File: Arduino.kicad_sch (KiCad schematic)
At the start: 1 part

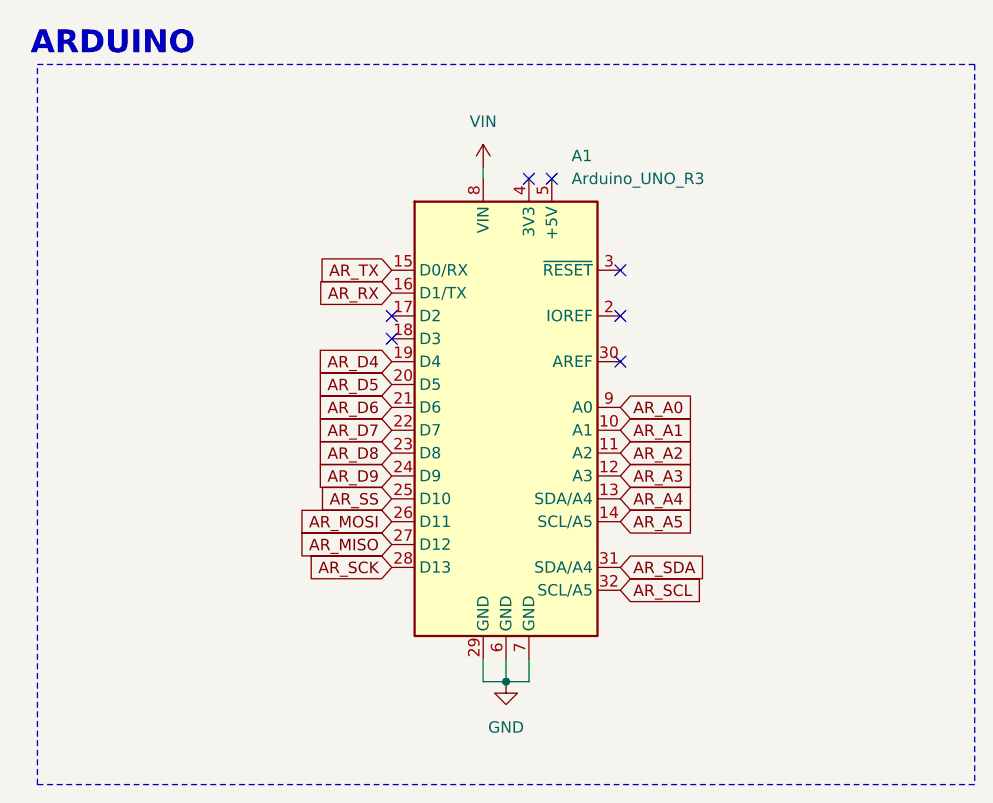
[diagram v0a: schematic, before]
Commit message: verification
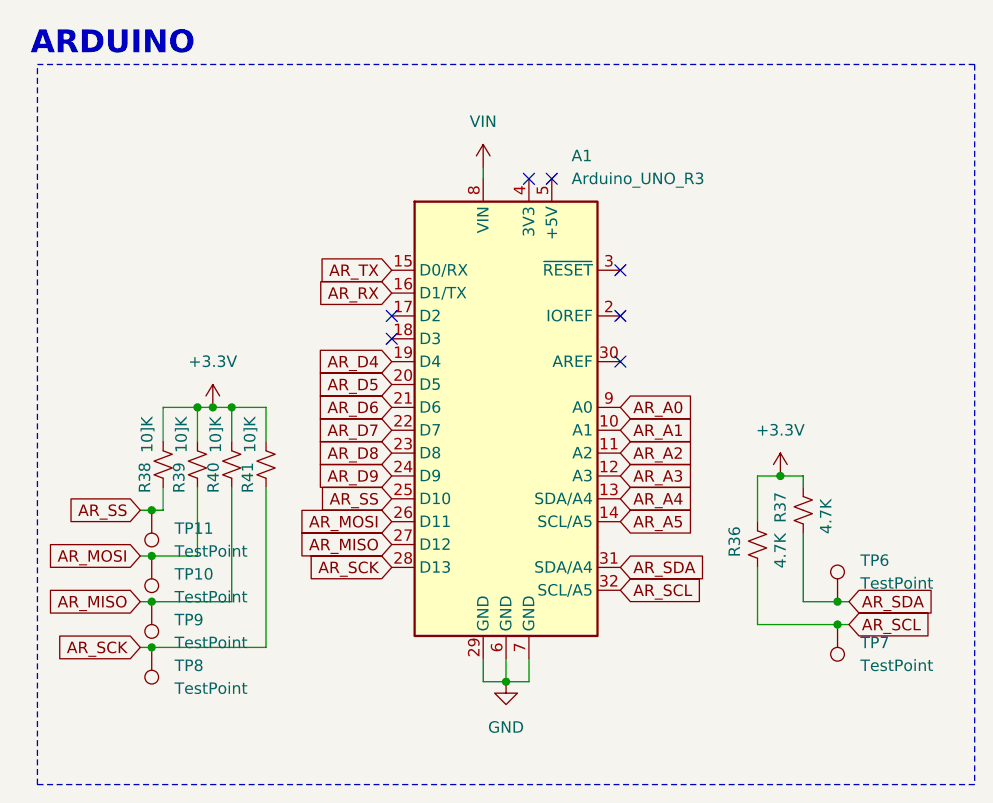
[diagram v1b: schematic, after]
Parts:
- added R36, R37: 4.7K, Resistor_SMD:R_0805_2012Metric, symbol Device:R_Small_US
- added R38, R39, R40, R41: 10]K, Resistor_SMD:R_0805_2012Metric, symbol Device:R_Small_US
- added TP10, TP11, TP6, TP7, TP8, TP9: TestPoint, TestPoint:TestPoint_Pad_D2.0mm, symbol Connector:TestPoint
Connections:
- net AR_MISO: now also R40.1, TP9.1
- net AR_MOSI: now also R39.1, TP10.1
- net AR_SCK: now also R41.1, TP8.1
- net AR_SCL: now also R36.1, TP7.1
- net AR_SDA: now also R37.1, TP6.1
- net AR_SS: now also R38.1, TP11.1
- new net +3.3V: R36.2, R37.2, R38.2, R39.2, R40.2, R41.2
